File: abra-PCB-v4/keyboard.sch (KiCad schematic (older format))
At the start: 165 parts, among them SW1 Rotary_Encoder_Switch

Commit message: added usb + mcu
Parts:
- added C?: C_Small, symbol Device:C_Small
- added J?: USB_C_Receptacle_USB2.0, symbol Connector:USB_C_Receptacle_USB2.0
- added R?: R_Small, symbol Device:R_Small
- added U?: ATmega32U4-AU, Package_QFP:TQFP-44_10x10mm_P0.8mm, symbol MCU_Microchip_ATmega:ATmega32U4-AU
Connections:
- net labels added: +5V, GND
- wire segments 336 -> 346
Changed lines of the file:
@@
 	7550 4550 7950 4550
 Connection ~ 7950 4550
+$Comp
+L MCU_Microchip_ATmega:ATmega32U4-AU U?
+U 1 1 5F1D63B5
+P 2350 6700
+F 0 "U?" H 2350 4811 50  0000 C CNN
+F 1 "ATmega32U4-AU" H 2350 4720 50  0000 C CNN
+F 2 "Package_QFP:TQFP-44_10x10mm_P0.8mm" H 2350 6700 50  0001 C CIN
+F 3 "http://ww1.microchip.com/downloads/en/DeviceDoc/Atmel-7766-8-bit-AVR-ATmega16U4-32U4_Datasheet.pdf" H 2350 6700 50  0001 C CNN
+	1    2350 6700
+	1    0    0    -1
+$EndComp
+$Comp
+L Connector:USB_C_Receptacle_USB2.0 J?
+U 1 1 5F1D7C40
+P 3250 11400
+F 0 "J?" H 3357 12267 50  0000 C CNN
+F 1 "USB_C_Receptacle_USB2.0" H 3357 12176 50  0000 C CNN
+F 2 "" H 3400 11400 50  0001 C CNN
+F 3 "https://www.usb.org/sites/default/files/documents/usb_type-c.zip" H 3400 11400 50  0001 C CNN
+	1    3250 11400
+	1    0    0    -1
+$EndComp
+$Comp
+L power:GND #PWR?
+U 1 1 5F1DA9CA
+P 2000 8500
+F 0 "#PWR?" H 2000 8250 50  0001 C CNN
+F 1 "GND" H 2005 8327 50  0000 C CNN
+F 2 "" H 2000 8500 50  0001 C CNN
+F 3 "" H 2000 8500 50  0001 C CNN
+	1    2000 8500
+	1    0    0    -1
+$EndComp
+Wire Wire Line
+	2350 8500 2250 8500
+Connection ~ 2250 8500
+Wire Wire Line
+	2250 8500 2000 8500
+$Comp
+L Device:R_Small R?
+U 1 1 5F1FB239
+P 3450 7300
+F 0 "R?" V 3254 7300 50  0000 C CNN
+F 1 "R_Small" V 3345 7300 50  0000 C CNN
+F 2 "" H 3450 7300 50  0001 C CNN
+F 3 "~" H 3450 7300 50  0001 C CNN
+	1    3450 7300
+	0    1    1    0
+$EndComp
+$Comp
+L power:GND #PWR?
+U 1 1 5F1FC218
+P 3950 7300
+F 0 "#PWR?" H 3950 7050 50  0001 C CNN
+F 1 "GND" H 3955 7127 50  0000 C CNN
+F 2 "" H 3950 7300 50  0001 C CNN
+F 3 "" H 3950 7300 50  0001 C CNN
+	1    3950 7300
+	1    0    0    -1
+$EndComp
+Wire Wire Line
+	2950 7300 3350 7300
+Wire Wire Line
+	3550 7300 3950 7300
+Wire Wire Line
+	1750 6500 1200 6500
+$Comp
+L Device:C_Small C?
+U 1 1 5F23DA59
+P 1200 6600
+F 0 "C?" H 1292 6646 50  0000 L CNN
+F 1 "C_Small" H 1292 6555 50  0000 L CNN
+F 2 "" H 1200 6600 50  0001 C CNN
+F 3 "~" H 1200 6600 50  0001 C CNN
+	1    1200 6600
+	1    0    0    -1
+$EndComp
+Wire Wire Line
+	1200 6700 1200 6900
+$Comp
+L power:GND #PWR?
+U 1 1 5F260633
+P 1200 6900
+F 0 "#PWR?" H 1200 6650 50  0001 C CNN
+F 1 "GND" H 1205 6727 50  0000 C CNN
+F 2 "" H 1200 6900 50  0001 C CNN
+F 3 "" H 1200 6900 50  0001 C CNN
+	1    1200 6900
+	1    0    0    -1
+$EndComp
+Wire Wire Line
+	2250 4900 2250 4650
+$Comp
+L power:+5V #PWR?
+U 1 1 5F28253C
+P 2250 4650
+F 0 "#PWR?" H 2250 4500 50  0001 C CNN
+F 1 "+5V" H 2265 4823 50  0000 C CNN
+F 2 "" H 2250 4650 50  0001 C CNN
+F 3 "" H 2250 4650 50  0001 C CNN
+	1    2250 4650
+	1    0    0    -1
+$EndComp
+Wire Wire Line
+	2250 4900 2350 4900
+Connection ~ 2250 4900
+Connection ~ 2350 4900
+Wire Wire Line
+	2350 4900 2450 4900
+Wire Wire Line
+	1750 6000 1550 6000
+$Comp
+L power:+5V #PWR?
+U 1 1 5F2E9291
+P 1550 6000
+F 0 "#PWR?" H 1550 5850 50  0001 C CNN
+F 1 "+5V" H 1565 6173 50  0000 C CNN
+F 2 "" H 1550 6000 50  0001 C CNN
+F 3 "" H 1550 6000 50  0001 C CNN
+	1    1550 6000
+	1    0    0    -1
+$EndComp
 $EndSCHEMATC

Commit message: updated schematic
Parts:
- added C1, C5, C6: 0.1uF, symbol Device:C_Small
- added C2, C3: 22pF, symbol Device:C_Small
- added C7: 10uF, symbol Device:C_Small
- added C8: 4.7uF, symbol Device:C_Small
- added F1: 500mA Hold, symbol Device:Polyfuse_Small
- added R1, R2: 22, symbol Device:R_Small
- added R3: 10k, symbol Device:R_Small
- added R4: 1M, symbol Device:R_Small
- added R6, R7: 5.1k, symbol Device:R_Small
- added SW2: SW_Push, symbol Switch:SW_Push
- added U2: PRTR5V0U2X, symbol random-keyboard-parts:PRTR5V0U2X
- added Y1: 16MHz, symbol Device:Crystal_GND24_Small
- C4: renamed from C?; value C_Small -> 1uF
- R5: renamed from R?; value R_Small -> 10k
- gave numbers to parts that had none: 2
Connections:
- net labels added: D+, D-, VCC
- wire segments 346 -> 423

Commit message: added underglow and backlighting
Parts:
- added C10, C11, C12, C13, C14, C15, C16, C17, C18, C19, C20, C9: 0.1uF, acheron_Components:C_0805_2012Metric, symbol Device:C_Small
- added D1, D10, D11, D12, D2, D3, D4, D5, D6, D7, D8, D9: WS2812B, LED_SMD:LED_WS2812B_PLCC4_5.0x5.0mm_P3.2mm, symbol LED:WS2812B
- added J2: Conn_2Rows-07Pins, symbol Connector_Generic:Conn_2Rows-07Pins
- added Q1: Q_NPN_BCE, symbol Device:Q_NPN_BCE
- added R10, R11, R12, R13, R14, R15, R16, R17, R18, R19, R20, R21, R22, R23, R24, R25, R26, R27, R28, R29, R30, R31, R32, R33, R34, R35, R36, R37, R38, R39, R40, R41, R42, R43, R44, R45, R46, R47, R48, R49, R50, R51, R52, R53, R54, R55, R56, R57, R58, R59, R60, R61, R62, R63, R64, R65, R66, R67, R68, R69, R70, R71, R72, R73, R74, R75, R76, R77, R78, R79, R80, R81, R82, R83, R84, R85, R86, R87, R88, R89, R90: R_Small, symbol Device:R_Small
- added R8: 500, symbol Device:R_Small
- added R9: 1.5k, symbol Device:R_Small
- C1, C2, C3, C4, C5, C6, C7, C8: footprint (none) -> acheron_Components:C_0805_2012Metric
- F1: footprint (none) -> acheron_Components:Fuse_1812_4532
- K_0, K_1, K_10, K_11, K_12, K_14, K_15, K_16, K_17, K_18, K_19, K_2, K_20, K_21, K_22, K_23, K_24, K_25, K_26, K_27, K_28, K_29, K_3, K_30, K_31, K_32, K_33, K_34, K_35, K_36, K_37, K_38, K_39, K_4, K_40, K_41, K_42, K_43, K_44, K_46, K_47, K_48, K_49, K_5, K_50, K_51, K_52, K_53, K_54, K_55, K_56, K_57, K_58, K_59, K_6, K_60, K_61, K_62, K_63, K_64, K_65, K_66, K_67, K_68, K_69, K_7, K_70, K_71, K_72, K_73, K_74, K_75, K_76, K_77, K_78, K_79, K_8, K_80, K_81, K_82, K_9: symbol MX_Alps_Hybrid:MX-NoLED -> MX_Alps_Hybrid:MX-LED
- K_45: value KEYSW -> MX-NoLED; footprint MX_Only:MXOnly-1.25U-NoLED -> MX_Only:MXOnly-1.75U-NoLED
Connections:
- net labels added: LEDGND, LEDPWM, MISO, MOSI, RGBIN, RST, SCK
- wire segments 423 -> 673
- no-connect marks 0 -> 2
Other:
- moved on the sheet: D_0, D_1, D_10, D_11, D_12, D_13, D_14, D_15, D_16, D_17, D_18, D_19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

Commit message: layout changes
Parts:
- removed J1: USB_C_Receptacle_USB2.0, symbol Connector:USB_C_Receptacle_USB2.0
- removed J2: Conn_2Rows-07Pins, symbol Connector_Generic:Conn_2Rows-07Pins
- added J2: Conn_01x04, Connector_PinHeader_2.54mm:PinHeader_1x04_P2.54mm_Vertical_SMD_Pin1Left, symbol Connector_Generic:Conn_01x04
- added P1: TC2030-AVR, Keebio-Parts:Header-6-Pin-ZigZag, symbol keebio:TC2030-AVR
- added R91, R92: 22, acheron_Components:R_SMD_1206, symbol Device:R_Small
- added USB1: HRO-TYPE-C-31-M-12, Type-C:HRO-TYPE-C-31-M-12-HandSoldering, symbol keebio:HRO-TYPE-C-31-M-12
- K_0, K_1, K_10, K_11, K_12, K_14, K_15, K_16, K_17, K_18, K_19, K_2, K_20, K_21, K_22, K_23, K_24, K_25, K_26, K_28, K_3, K_30, K_31, K_32, K_33, K_34, K_35, K_36, K_37, K_38, K_39, K_4, K_40, K_41, K_43, K_46, K_47, K_48, K_49, K_5, K_50, K_51, K_52, K_53, K_54, K_55, K_56, K_58, K_6, K_60, K_61, K_62, K_63, K_64, K_65, K_66, K_67, K_68, K_69, K_7, K_71, K_72, K_77, K_78, K_79, K_8, K_80, K_81, K_82, K_9: footprint MX_Only:MXOnly-1U-NoLED -> MX_Only:MXOnly-1U
- K_27: footprint MX_Only:MXOnly-2U-NoLED -> MX_Only:MXOnly-2U
- K_29, K_42: footprint MX_Only:MXOnly-1.5U-NoLED -> MX_Only:MXOnly-1.5U
- K_44, K_70: footprint MX_Only:MXOnly-1.75U-NoLED -> MX_Only:MXOnly-1.75U
- K_57, K_59: footprint MX_Only:MXOnly-2.25U-NoLED -> MX_Only:MXOnly-2.25U
- K_73, K_74, K_75: footprint MX_Only:MXOnly-1.25U-NoLED -> MX_Only:MXOnly-1.25U
- K_76: footprint MX_Only:MXOnly-6.25U-NoLED -> MX_Only:MXOnly-6.25U
- Q1: footprint (none) -> Package_TO_SOT_SMD:SOT-223-3_TabPin2
- R1, R10, R11, R12, R13, R14, R15, R16, R17, R18, R19, R2, R20, R21, R22, R23, R24, R25, R26, R27, R28, R29, R3, R30, R31, R32, R33, R34, R35, R36, R37, R38, R39, R4, R40, R41, R42, R43, R44, R45, R46, R47, R48, R49, R5, R50, R51, R52, R53, R54, R55, R56, R57, R58, R59, R6, R60, R61, R62, R63, R64, R65, R66, R67, R68, R69, R7, R70, R71, R72, R73, R74, R75, R76, R77, R78, R79, R8, R80, R81, R82, R83, R84, R85, R86, R87, R88, R89, R9, R90: footprint (none) -> acheron_Components:R_SMD_1206
- SW2: footprint (none) -> random-keyboard-parts:Reset_Pretty
- U2: footprint (none) -> Nexperia:SOT143B
- Y1: footprint (none) -> Keebio-Parts:Crystal_SMD_3225-4pin_3.2x2.5mm
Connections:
- wire segments 673 -> 695
- no-connect marks 2 -> 3
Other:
- moved on the sheet: C8, F1, R4, R6, R7

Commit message: layout updates
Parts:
- added R93: R_Small, acheron_Components:R_SMD_1206, symbol Device:R_Small
- K_45: footprint MX_Only:MXOnly-1.75U-NoLED -> MX_Only:MXOnly-1.75U; symbol MX_Alps_Hybrid:MX-NoLED -> MX_Alps_Hybrid:MX-LED
- P1: symbol keebio:TC2030-AVR -> keyboard-rescue:TC2030-AVR-keebio
- U2: symbol random-keyboard-parts:PRTR5V0U2X -> keyboard-rescue:PRTR5V0U2X-random-keyboard-parts
- USB1: symbol keebio:HRO-TYPE-C-31-M-12 -> keyboard-rescue:HRO-TYPE-C-31-M-12-keebio
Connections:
- wire segments 695 -> 697
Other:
- moved on the sheet: R21

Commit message: light fix + library update
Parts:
- removed C19, C20: 0.1uF, acheron_Components:C_0805_2012Metric, symbol Device:C_Small
- removed D1, D10, D11, D12, D2, D3, D4, D5, D6, D7, D8, D9: WS2812B, LED_SMD:LED_WS2812B_PLCC4_5.0x5.0mm_P3.2mm, symbol LED:WS2812B
- added D1, D10, D2, D3, D4, D5, D6, D7, D8, D9: SK6805, LED_SMD:LED_SK6812_EC15_1.5x1.5mm, symbol LED:SK6805
- U1: symbol MCU_Microchip_ATmega:ATmega32U4-AU -> keyboard-rescue:ATmega32U4-AU-MCU_Microchip_ATmega
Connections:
- net +5V: now also D1.4 (VDD), D10.4 (VDD), D2.4 (VDD), D3.4 (VDD), D4.4 (VDD), D5.4 (VDD), D6.4 (VDD), D7.4 (VDD), D8.4 (VDD), D9.4 (VDD)
- net GND: now also D1.2 (VSS), D10.2 (VSS), D2.2 (VSS), D3.2 (VSS), D4.2 (VSS), D5.2 (VSS), D6.2 (VSS), D7.2 (VSS), D8.2 (VSS), D9.2 (VSS)
- net at R8.1: now also D1.3 (DIN)
- new net: D1.1 (DOUT), D2.3 (DIN)
- new net: D2.1 (DOUT), D3.3 (DIN)
- new net: D3.1 (DOUT), D4.3 (DIN)
- new net: D4.1 (DOUT), D5.3 (DIN)
- new net: D5.1 (DOUT), D6.3 (DIN)
- new net: D6.1 (DOUT), D7.3 (DIN)
- new net: D7.1 (DOUT), D8.3 (DIN)
- new net: D8.1 (DOUT), D9.3 (DIN)
- new net: D10.3 (DIN), D9.1 (DOUT)
- no-connect marks 3 -> 2
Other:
- moved on the sheet: C10, C11, C12, C13, C14, C15, C16, C17, C18, C8, C9, F1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

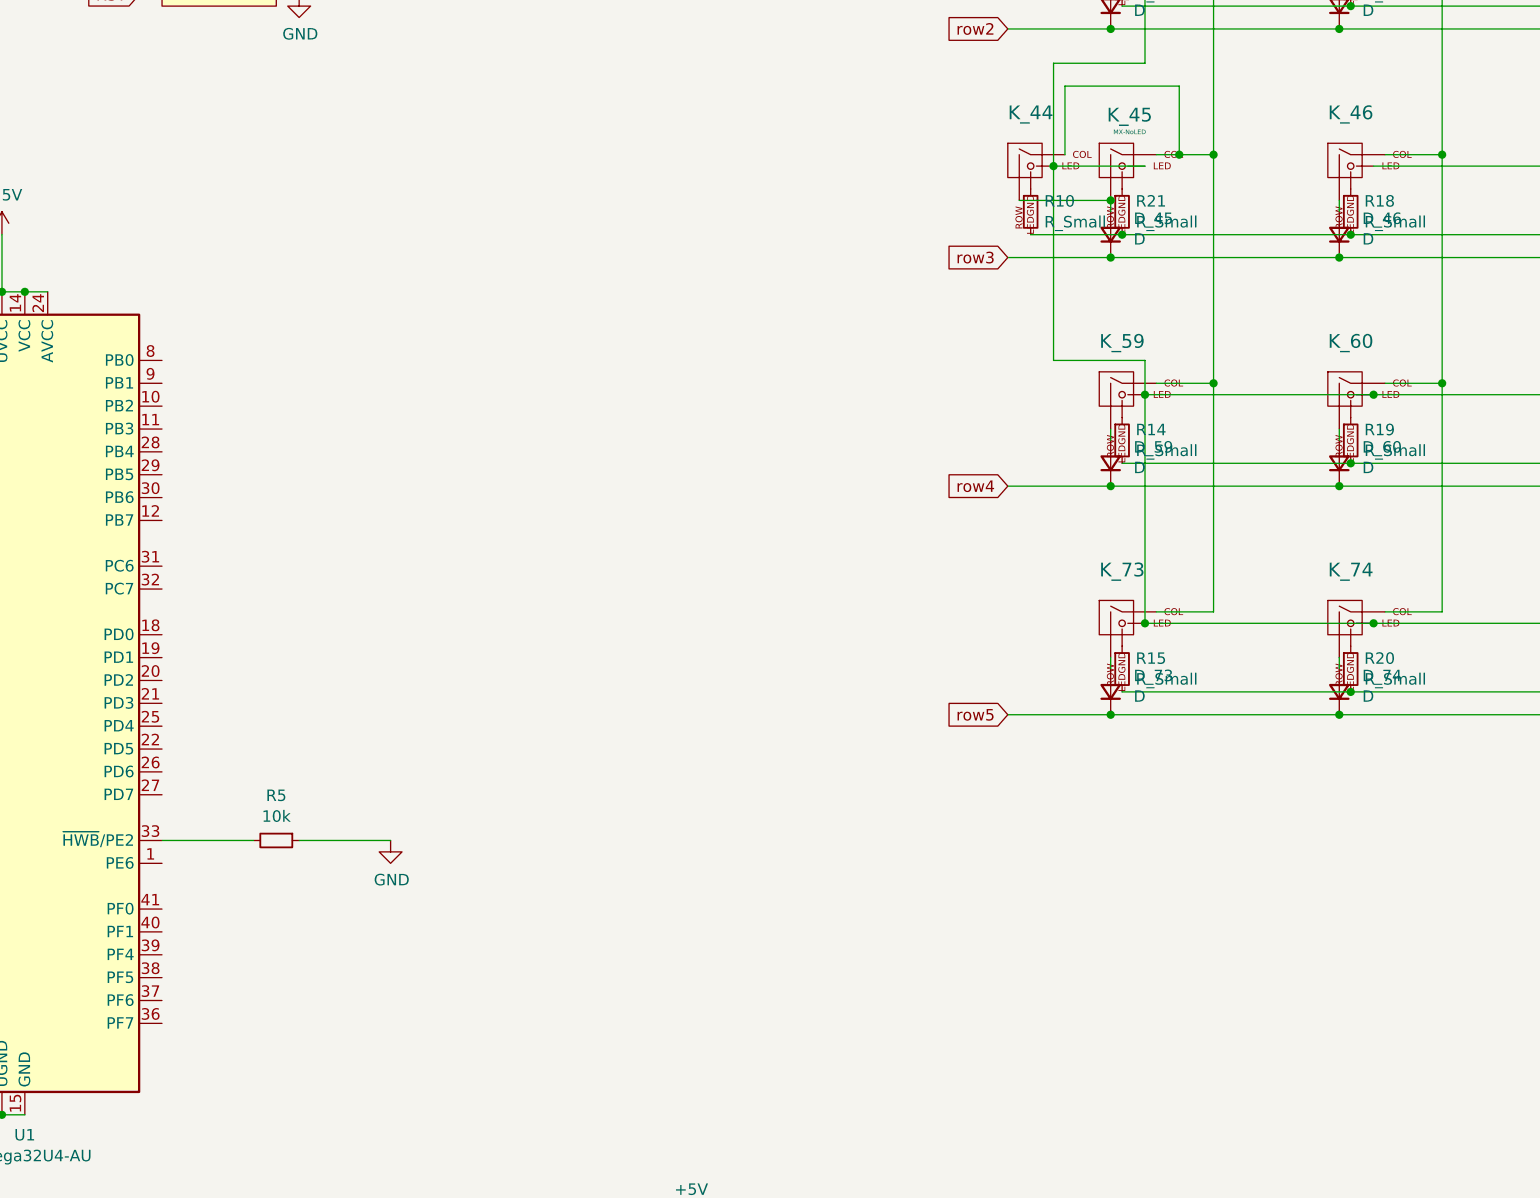
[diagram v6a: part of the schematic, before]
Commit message: routing updates
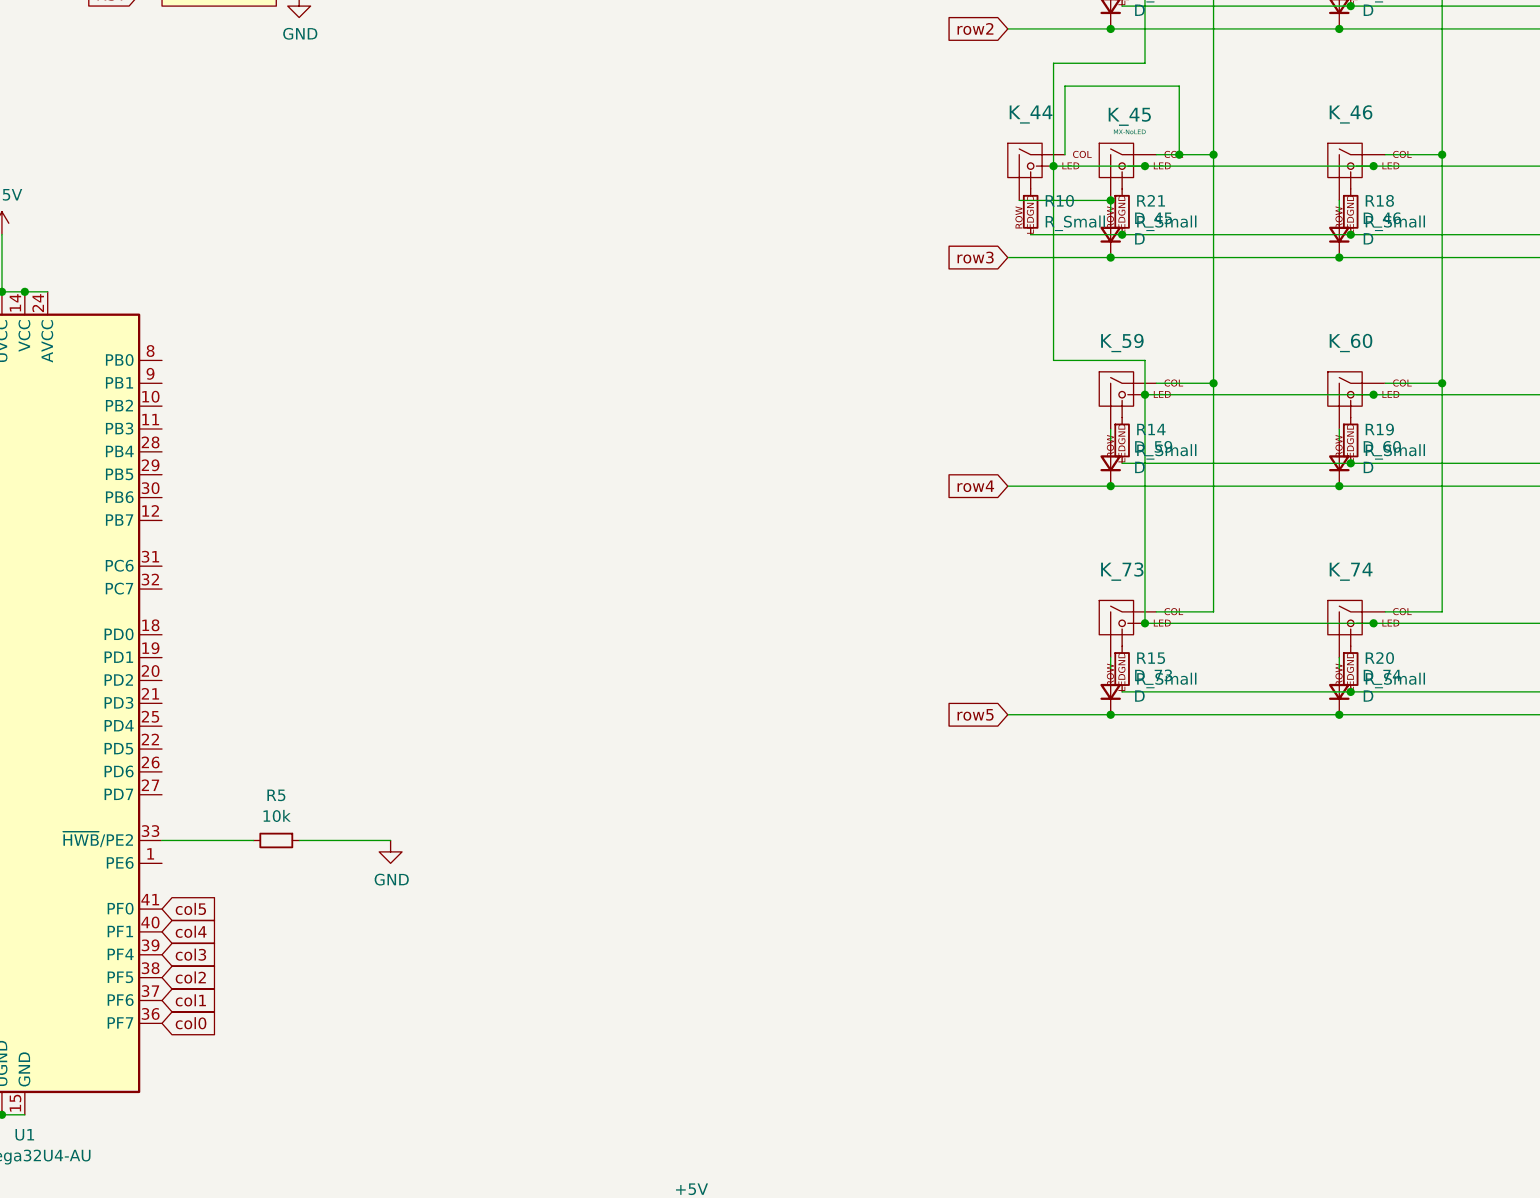
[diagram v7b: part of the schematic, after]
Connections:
- net +5V: now also K_46.3 (LED), K_47.3 (LED), K_48.3 (LED), K_49.3 (LED), K_50.3 (LED), K_51.3 (LED), K_52.3 (LED), K_53.3 (LED), K_54.3 (LED), K_55.3 (LED), K_56.3 (LED), K_57.3 (LED), K_58.3 (LED)
- net col0: now also U1.36 (PF7)
- net col1: now also U1.37 (PF6)
- net col2: now also U1.38 (PF5)
- net col3: now also U1.39 (PF4)
- net col4: now also U1.40 (PF1)
- net col5: now also U1.41 (PF0)
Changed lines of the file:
@@
 	7250 5200 7250 5350
 Connection ~ 6850 4350
-$Comp
-L MX_Alps_Hybrid:MX-LED K_45
-U 1 1 6219926C
-P 7150 4350
-F 0 "K_45" H 7183 4573 60  0000 C CNN
-F 1 "MX-NoLED" H 7183 4499 20  0000 C CNN
-F 2 "MX_Only:MXOnly-1.75U" H 6525 4325 60  0001 C CNN
-F 3 "" H 6525 4325 60  0001 C CNN
-	1    7150 4350
-	1    0    0    -1
-$EndComp
-Connection ~ 7100 4500
 Wire Wire Line
 	20150 1650 19150 1650
@@
 Connection ~ 9050 10400
 Connection ~ 9450 10400
+Text GLabel 2950 8100 2    50   Input ~ 0
+col0
+Text GLabel 2950 8000 2    50   Input ~ 0
+col1
+Text GLabel 2950 7900 2    50   Input ~ 0
+col2
+Text GLabel 2950 7800 2    50   Input ~ 0
+col3
+Text GLabel 2950 7700 2    50   Input ~ 0
+col4
+Text GLabel 2950 7600 2    50   Input ~ 0
+col5
+Connection ~ 7100 4500
+$Comp
+L MX_Alps_Hybrid:MX-LED K_45
+U 1 1 6219926C
+P 7150 4350
+F 0 "K_45" H 7183 4573 60  0000 C CNN
+F 1 "MX-NoLED" H 7183 4499 20  0000 C CNN
+F 2 "MX_Only:MXOnly-1.75U" H 6525 4325 60  0001 C CNN
+F 3 "" H 6525 4325 60  0001 C CNN
+	1    7150 4350
+	1    0    0    -1
+$EndComp
+Wire Wire Line
+	7250 4350 8250 4350
+Connection ~ 7250 4350
+Connection ~ 8250 4350
 $EndSCHEMATC
